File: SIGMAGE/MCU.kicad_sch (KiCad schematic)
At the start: 22 parts, among them U8 STM32F407VGTx, X1 STDCSU18M

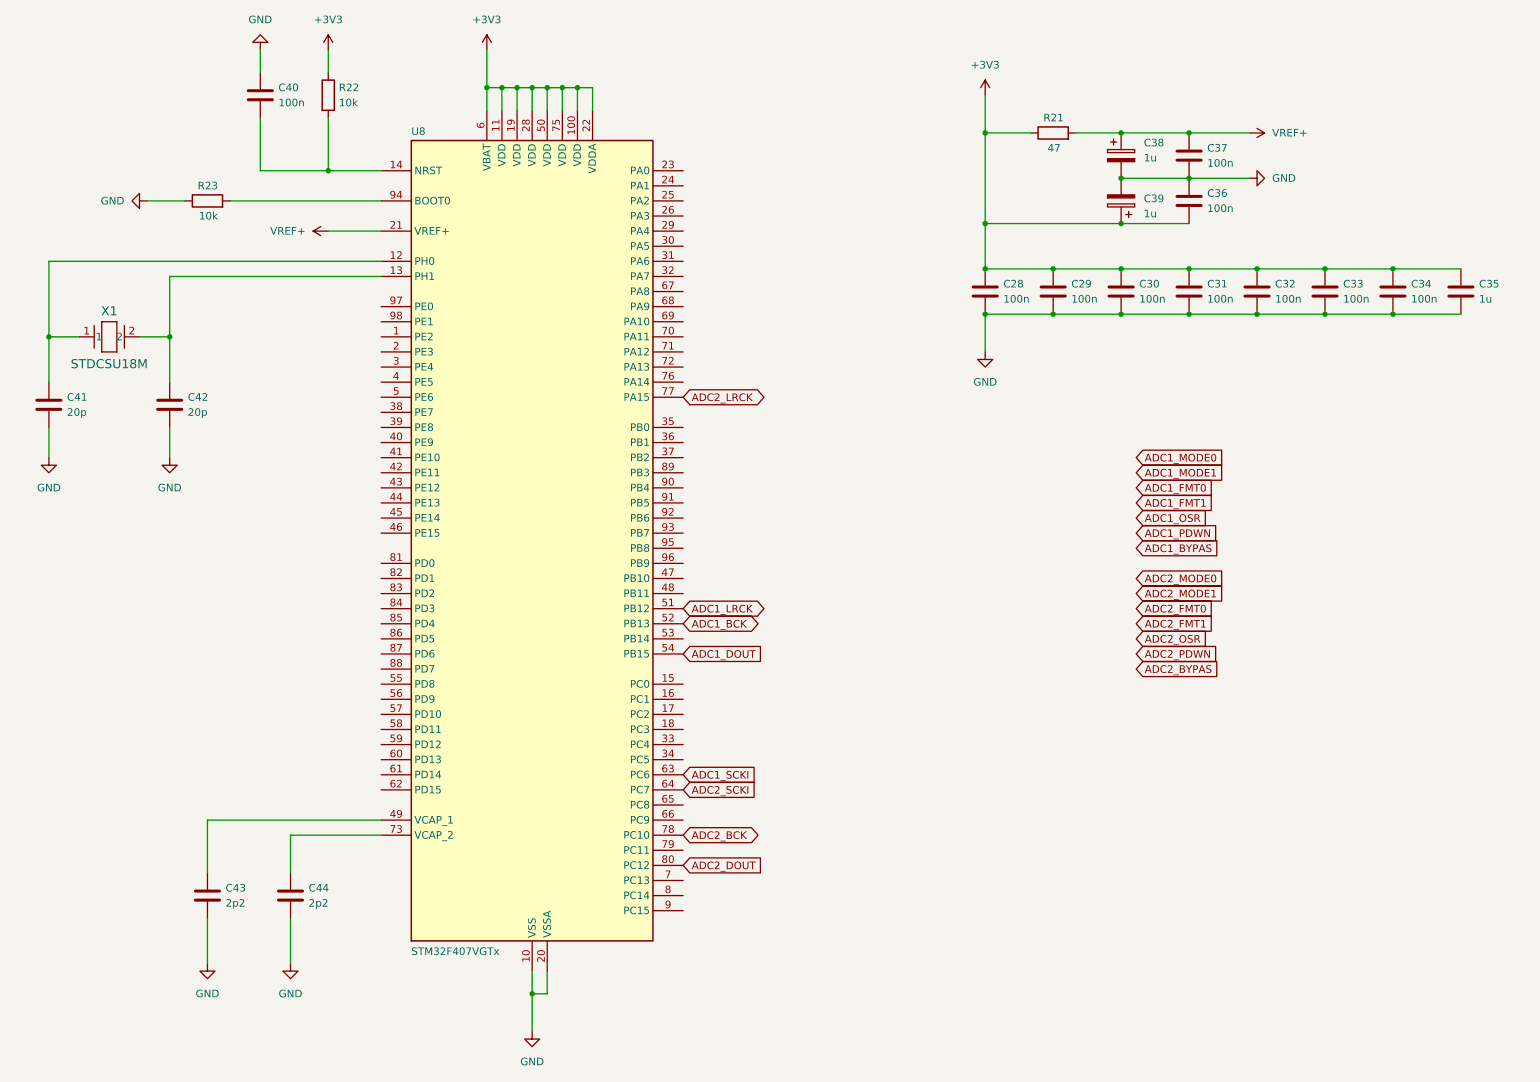
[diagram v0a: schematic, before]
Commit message: Finished schematic
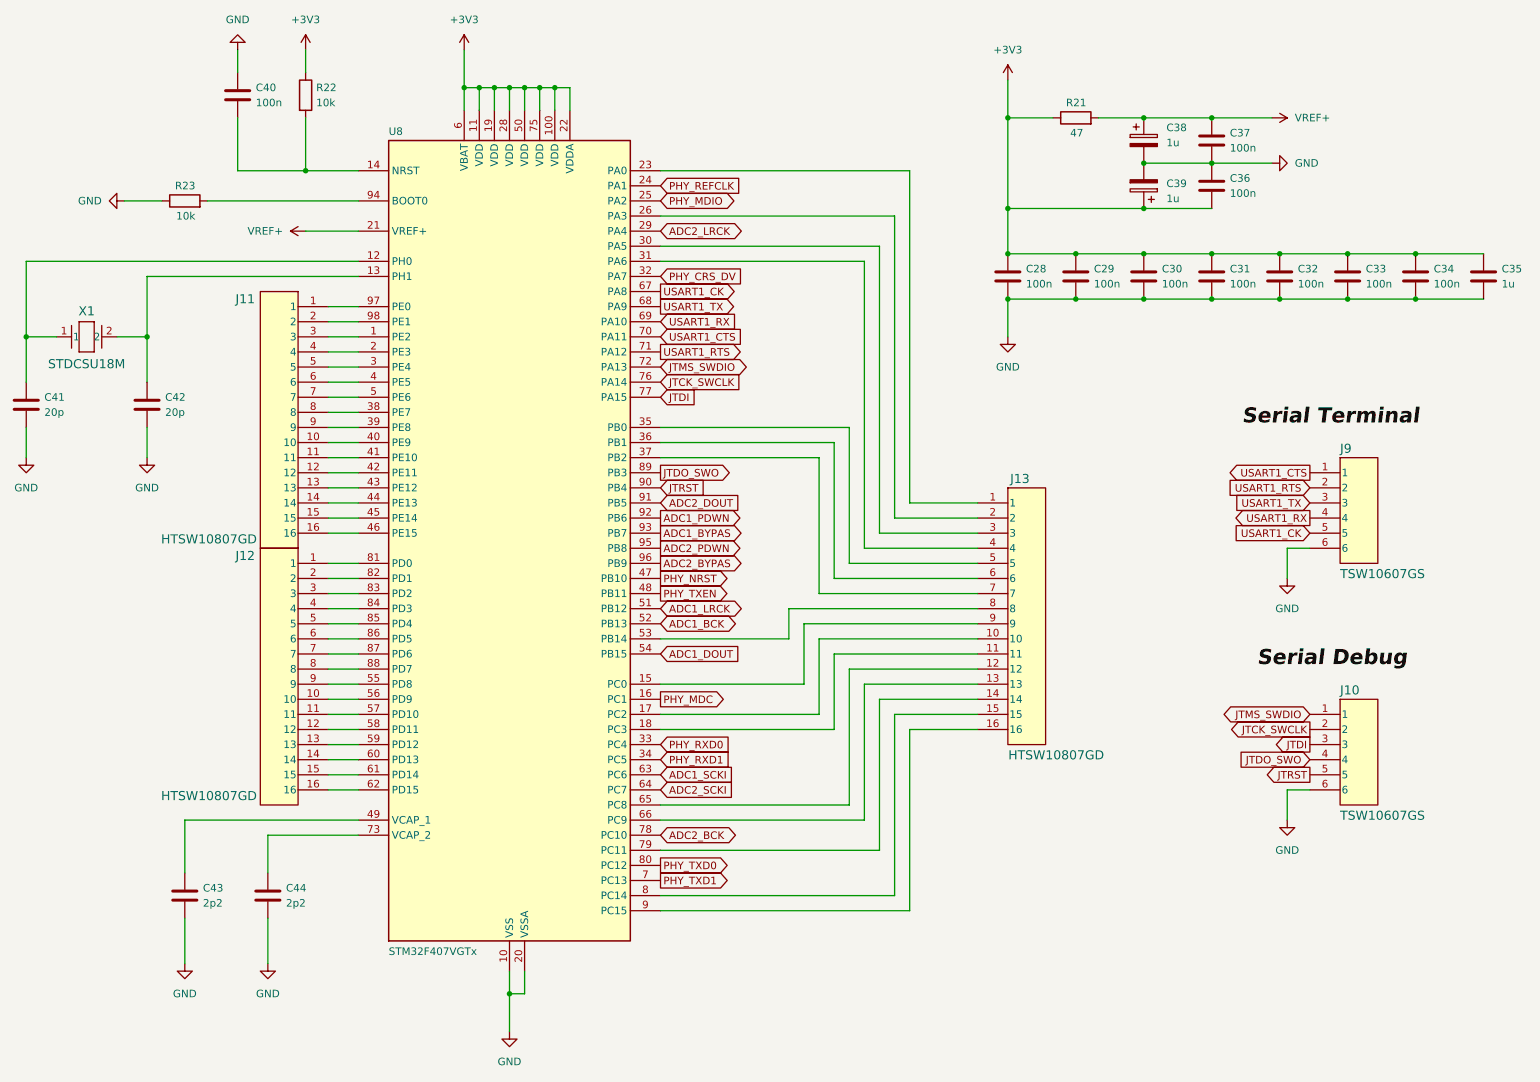
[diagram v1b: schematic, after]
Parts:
- added J10, J9: TSW10607GS, SIGMAGE:TSW10607GS, symbol SIGMAGE:TSW10607GS
- added J11, J12, J13: HTSW10807GD, SIGMAGE:HTSW10807GD, symbol SIGMAGE:HTSW10807GD
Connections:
- net ADC1_BYPAS: now also U8.93 (PB7)
- net ADC1_PDWN: now also U8.92 (PB6)
- net ADC2_BYPAS: now also U8.96 (PB9)
- net ADC2_DOUT: now also U8.91 (PB5); no longer U8.80 (PC12)
- net ADC2_LRCK: now also U8.29 (PA4); no longer U8.77 (PA15)
- net ADC2_PDWN: now also U8.95 (PB8)
- net GND: now also J10.6, J9.6
- net at U8.1 (PE2): now also J11.3
- net at U8.15 (PC0): now also J13.9
- net PHY_MDC: now reaches U8.16 (PC1)
- net at U8.17 (PC2): now also J13.10
- net at U8.18 (PC3): now also J13.11
- net at U8.2 (PE3): now also J11.4
- net at U8.23 (PA0): now also J13.1
- net PHY_REFCLK: now reaches U8.24 (PA1)
- net PHY_MDIO: now reaches U8.25 (PA2)
- net at U8.26 (PA3): now also J13.2
- net at U8.3 (PE4): now also J11.5
- net at U8.30 (PA5): now also J13.3
- net at U8.31 (PA6): now also J13.4
- net PHY_CRS_DV: now reaches U8.32 (PA7)
- net PHY_RXD0: now reaches U8.33 (PC4)
- net PHY_RXD1: now reaches U8.34 (PC5)
- net at U8.35 (PB0): now also J13.5
- net at U8.36 (PB1): now also J13.6
- net at U8.37 (PB2): now also J13.7
- net at U8.38 (PE7): now also J11.8
- net at U8.39 (PE8): now also J11.9
- net at U8.4 (PE5): now also J11.6
- net at U8.40 (PE9): now also J11.10
- net at U8.41 (PE10): now also J11.11
- net at U8.42 (PE11): now also J11.12
- net at U8.43 (PE12): now also J11.13
- net at U8.44 (PE13): now also J11.14
- net at U8.45 (PE14): now also J11.15
- net at U8.46 (PE15): now also J11.16
- net PHY_NRST: now reaches U8.47 (PB10)
- net PHY_TXEN: now reaches U8.48 (PB11)
- net at U8.5 (PE6): now also J11.7
- net at U8.53 (PB14): now also J13.8
- net at U8.55 (PD8): now also J12.9
- net at U8.56 (PD9): now also J12.10
- net at U8.57 (PD10): now also J12.11
- net at U8.58 (PD11): now also J12.12
- net at U8.59 (PD12): now also J12.13
- net at U8.60 (PD13): now also J12.14
- net at U8.61 (PD14): now also J12.15
- net at U8.62 (PD15): now also J12.16
- net at U8.65 (PC8): now also J13.12
- net at U8.66 (PC9): now also J13.13
- net USART1_CK: now reaches U8.67 (PA8)
- net USART1_CK: now also J9.5
- net USART1_TX: now reaches U8.68 (PA9)
- net USART1_TX: now also J9.3
- net USART1_RX: now reaches U8.69 (PA10)
- net USART1_RX: now also J9.4
- net PHY_TXD1: now reaches U8.7 (PC13)
- net USART1_CTS: now reaches U8.70 (PA11)
- net USART1_CTS: now also J9.1
- net USART1_RTS: now reaches U8.71 (PA12)
- net USART1_RTS: now also J9.2
- net JTMS_SWDIO: now reaches U8.72 (PA13)
- net JTMS_SWDIO: now also J10.1
- net JTCK_SWCLK: now reaches U8.76 (PA14)
- net JTCK_SWCLK: now also J10.2
- net at U8.79 (PC11): now also J13.14
- net at U8.8 (PC14): now also J13.15
- net at U8.81 (PD0): now also J12.1
- net at U8.82 (PD1): now also J12.2
- net at U8.83 (PD2): now also J12.3
- net at U8.84 (PD3): now also J12.4
- net at U8.85 (PD4): now also J12.5
- net at U8.86 (PD5): now also J12.6
- net at U8.87 (PD6): now also J12.7
- net at U8.88 (PD7): now also J12.8
- net JTDO_SWO: now reaches U8.89 (PB3)
- net JTDO_SWO: now also J10.4
- net at U8.9 (PC15): now also J13.16
- net JTRST: now reaches U8.90 (PB4)
- net JTRST: now also J10.5
- net at U8.97 (PE0): now also J11.1
- net at U8.98 (PE1): now also J11.2
- new net JTDI: J10.3, U8.77 (PA15)
- new net PHY_TXD0: U8.80 (PC12)
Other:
- moved on the sheet: C28, C29, C30, C31, C32, C33, C34, C35, C36, C37, C38, C39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
